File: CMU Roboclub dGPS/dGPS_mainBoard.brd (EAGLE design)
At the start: 95.3 x 74.9 mm, 15 parts, among them IC1 LM2937

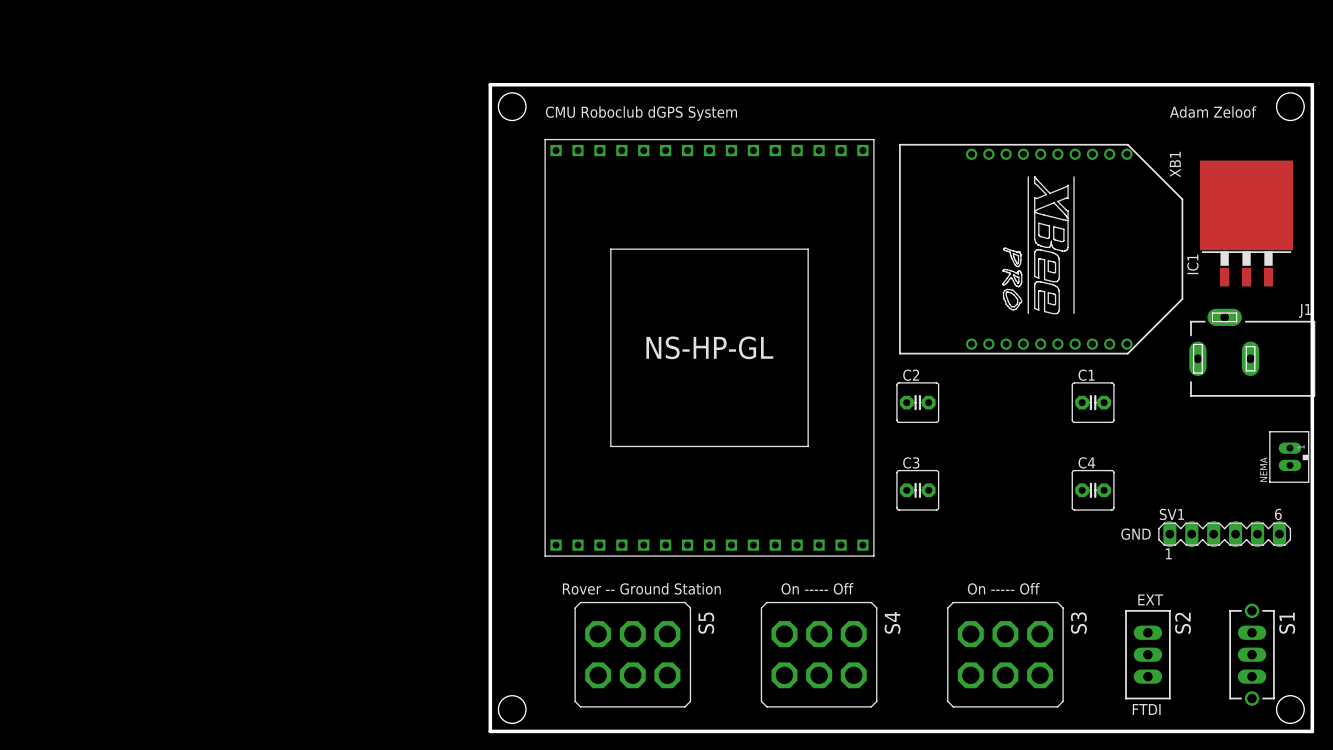
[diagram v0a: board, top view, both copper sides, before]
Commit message: Changed many things
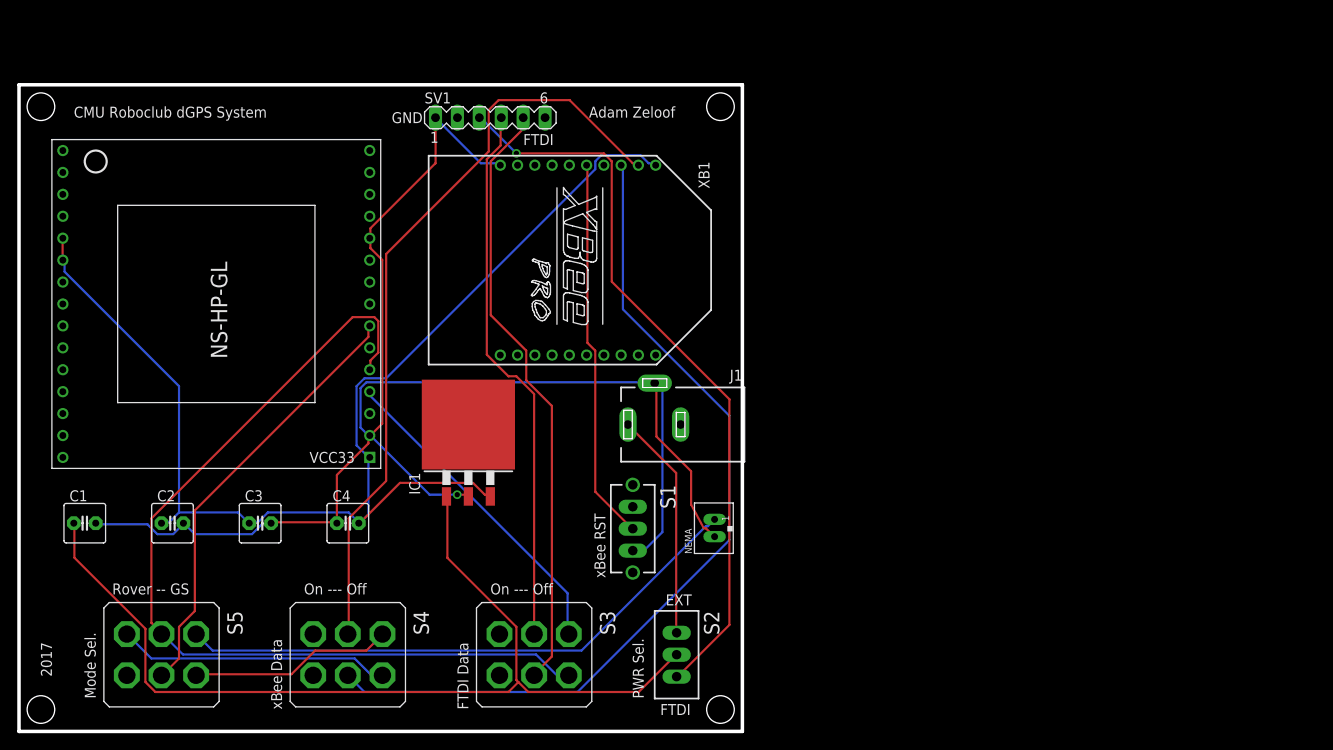
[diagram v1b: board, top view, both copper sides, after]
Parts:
- moved C1 117.7 mm to (7.62, 24.1)
- moved SV1 97.8 mm to (54.6, 71.1)
- moved IC1 93.7 mm to (52.1, 33.0)
- moved C2 87.5 mm to (17.8, 24.1)
- moved C4 86.4 mm to (38.1, 24.1)
- moved C3 76.3 mm to (27.9, 24.1)
- moved S1 73.2 mm to (71.1, 23.5)
- moved NEMA 67.2 mm to (80.6, 23.5)
- moved U$1 66.9 mm to (41.9, 30.5), turned to 0 degrees
- moved J1 66.5 mm to (73.7, 35.6)
- moved XB1 54.6 mm to (64.8, 54.6)
- moved S2 54.6 mm to (76.2, 8.89)
- moved S3 54.6 mm to (59.7, 8.89)
- moved S5 54.6 mm to (16.5, 8.89)
- moved S4 54.6 mm to (38.1, 8.89)
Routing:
- net N$12: track 0.00 -> 190.4 mm, vias 0 -> 1
- net N$1: track 0.00 -> 144.0 mm
- net N$15: track 0.00 -> 111.6 mm
- net N$9: track 0.00 -> 105.2 mm
- net N$10: track 0.00 -> 101.1 mm
- net N$11: track 0.00 -> 88.4 mm
- net N$16: track 0.00 -> 85.4 mm, vias 0 -> 1
- net N$2: track 0.00 -> 70.0 mm
- net N$7: track 0.00 -> 67.2 mm
- net N$8: track 0.00 -> 63.4 mm
- net N$3: track 0.00 -> 50.5 mm
- net N$13: track 0.00 -> 44.4 mm
- net N$4: track 0.00 -> 37.6 mm
- net N$6: track 0.00 -> 31.6 mm
- net N$14: track 0.00 -> 26.5 mm
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- added copper zone on layer 1, net N$17
- added copper zone on layer 16, net N$18
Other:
- board size 95.3 x 74.9 mm -> 83.8 x 74.9 mm
- board text added: "FTDI Data"
- board text added: "Mode Sel."
- board text added: "On --- Off"
- board text added: "PWR Sel."
- board text added: "Rover -- GS"
- board text added: "xBee Data"
- board text added: "xBee RST"
- board text removed: "On ----- Off"
- board text removed: "Rover -- Ground Station"

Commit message: Added indicator LEDs and did other stuff
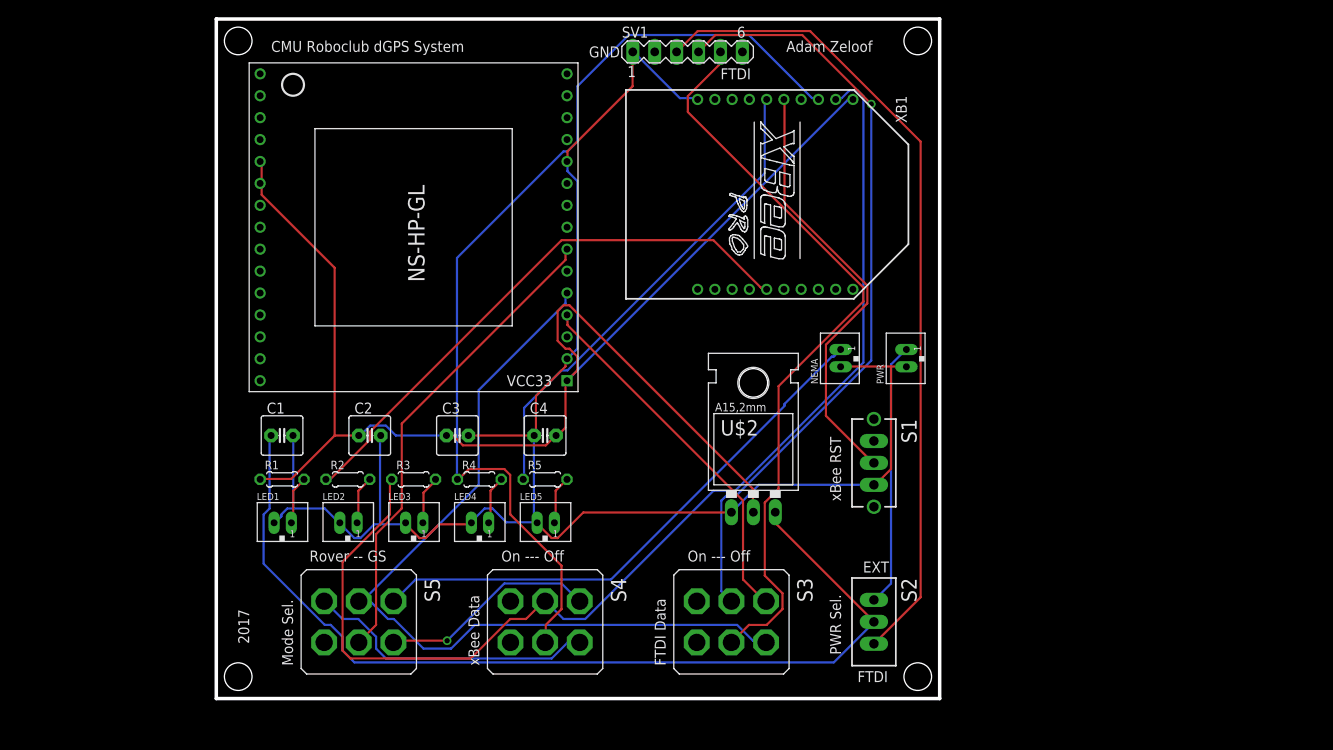
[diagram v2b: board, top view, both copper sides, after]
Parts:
- removed IC1: LM2937, linear:TO263-3
- removed J1: (no value), con-jack:DCJ0303
- added LED1: PWR, SRG:JST_B2B-PH_HEADER
- added LED2: xBee Assoc., SRG:JST_B2B-PH_HEADER
- added LED3: xBee RX, SRG:JST_B2B-PH_HEADER
- added LED4: xBee TX, SRG:JST_B2B-PH_HEADER
- added LED5: xBee RX Strength, SRG:JST_B2B-PH_HEADER
- added PWR: (no value), SRG:JST_B2B-PH_HEADER
- added R1, R2, R3, R4, R5: 1k, rcl:0204/5
- added U$2: LD1117V33, LD1117V33:LD1117V33
- moved S1 29.0 mm to (99.1, 31.1)
- moved C1 25.0 mm to (30.5, 34.3)
- moved C2 25.0 mm to (40.6, 34.3)
- moved C4 25.0 mm to (61.0, 34.3)
- moved C3 25.0 mm to (50.8, 34.3)
- moved U$1 24.5 mm to (64.8, 39.4)
- moved NEMA 24.5 mm to (95.2, 43.2)
- moved SV1 24.1 mm to (77.5, 78.7)
- moved XB1 24.1 mm to (87.6, 62.2)
- moved S2 23.2 mm to (99.1, 12.7)
- moved S3 23.2 mm to (82.5, 12.7)
- moved S4 23.2 mm to (61.0, 12.7)
- moved S5 23.2 mm to (39.4, 12.7)
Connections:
- new net N$17: C1.2, C2.2, C3.2, C4.1, LED1.P2, LED2.P2, LED3.P2, LED4.P2, LED5.P2, NEMA.P2, PWR.P2, S1.3, SV1.1, U$1.11, U$1.2, U$2.GND, XB1.10
- new net N$18: R5.1, XB1.6
- new net N$19: LED1.P1, R1.2
- new net N$20: LED2.P1, R2.2
- new net N$21: LED3.P1, R3.2
- new net N$22: LED4.P1, R4.2
- new net N$23: LED5.P1, R5.2
- net N$1: now also R1.1, U$2.OUT; no longer IC1.3
- net N$10: now also R4.1
- net N$11: now also R3.1
- net N$12: now also R2.1, XB1.15; no longer C1.2, C2.2, C3.2, C4.1, IC1.2, J1.2, NEMA.P2, S1.3, SV1.1, U$1.11, U$1.2, XB1.10
- net N$14: now also PWR.P1; no longer J1.1
- net N$15: now also U$2.IN; no longer IC1.1
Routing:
- net N$17: track 0.00 -> 198.1 mm
- net N$12: track 190.4 -> 65.4 mm, vias 1 -> 0
- net N$18: track 0.00 -> 56.2 mm
- net N$11: track 88.4 -> 133.7 mm
- net N$1: track 144.0 -> 171.6 mm
- net N$8: track 63.4 -> 90.1 mm, vias 0 -> 1
- net N$2: track 70.0 -> 87.7 mm
- net N$10: track 101.1 -> 114.7 mm
- net N$16: track 85.4 -> 95.0 mm, vias 1 -> 0
- net N$9: track 105.2 -> 97.8 mm
- net N$13: track 44.4 -> 50.5 mm
- net N$19: track 0.00 -> 5.71 mm
- net N$22: track 0.00 -> 5.71 mm
- net N$23: track 0.00 -> 5.68 mm
- net N$20: track 0.00 -> 5.68 mm
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- removed copper zone on layer 1, net N$17
- removed copper zone on layer 16, net N$18
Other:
- board size 83.8 x 74.9 mm -> 83.8 x 78.7 mm
